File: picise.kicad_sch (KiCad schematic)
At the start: 116 parts, among them J1 ANT_SMA, J2 SSQ-120-03_GPIO, J3 TSM-103-01-L-SV, U1 MAX-M10S, U2 PCA9557PW, U3 CAT24C256, U4 IS31FL3731-QF

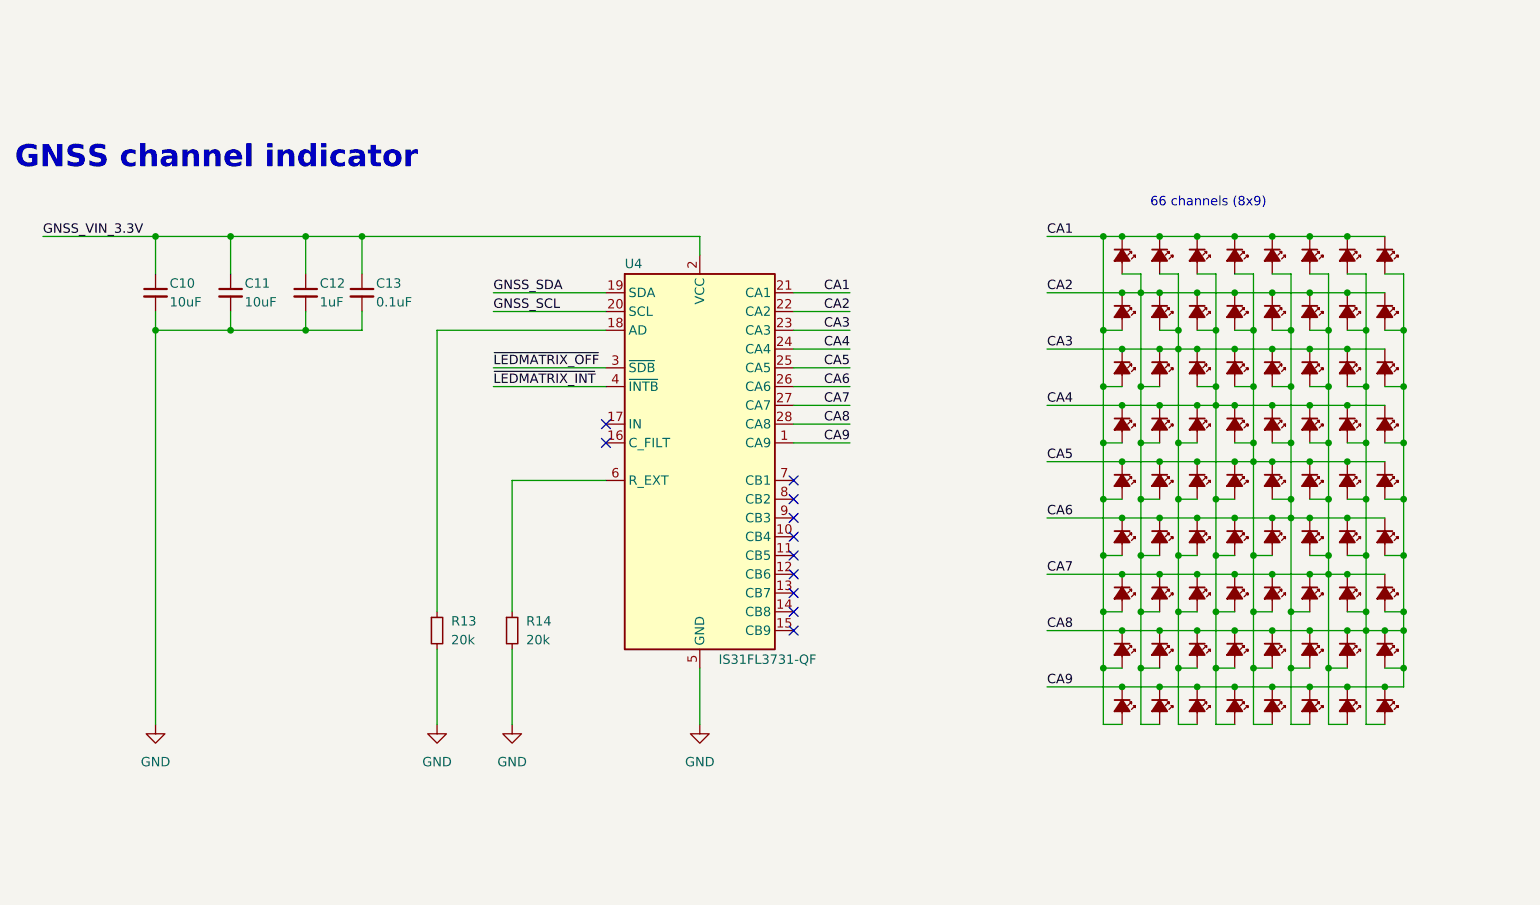
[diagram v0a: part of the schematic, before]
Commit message: rev2 prep
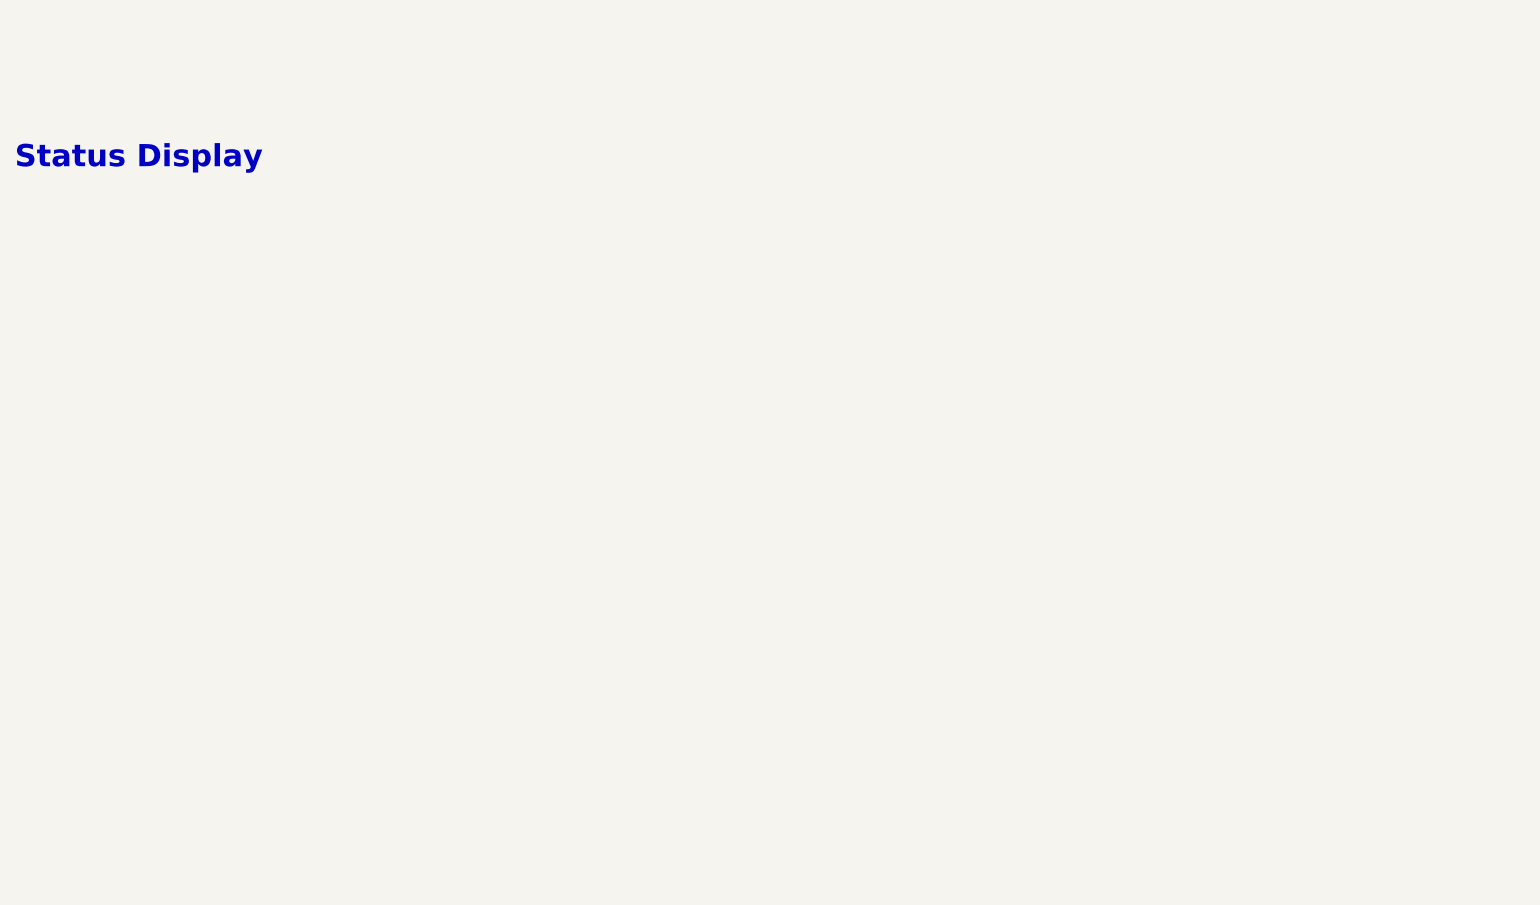
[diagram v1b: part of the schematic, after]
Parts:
- removed C10, C11: 10uF, Capacitor_SMD:C_0603_1608Metric, symbol Device:C_Small
- removed C12: 1uF, Capacitor_SMD:C_0603_1608Metric, symbol Device:C_Small
- removed C13: 0.1uF, Capacitor_SMD:C_0603_1608Metric, symbol Device:C_Small
- removed D1, D10, D11, D12, D13, D14, D15, D16, D17, D18, D19, D2, D20, D21, D22, D23, D24, D26, D27, D28, D29, D3, D30, D31, D32, D33, D34, D35, D36, D37, D38, D39, D4, D40, D41, D43, D44, D45, D46, D47, D48, D49, D5, D50, D51, D52, D53, D54, D55, D56, D57, D58, D59, D6, D60, D61, D62, D63, D64, D65, D66, D67, D68, D7, D70, D71, D72, D73, D74, D75, D8, D9: Green, Diode_SMD:D_0603_1608Metric, symbol Device:LED_Small_Filled
- removed R13, R14: 20k, Resistor_SMD:R_0603_1608Metric, symbol Device:R_Small
- removed U4: IS31FL3731-QF, Package_DFN_QFN:QFN-28-1EP_4x4mm_P0.4mm_EP2.3x2.3mm, symbol Driver_LED:IS31FL3731-QF
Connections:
- no-connect marks 21 -> 10
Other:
- note added: "Status Display"
- note removed: "66 channels (8x9)"
- note removed: "GNSS channel indicator"
